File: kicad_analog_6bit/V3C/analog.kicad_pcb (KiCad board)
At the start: 2 copper layers, 50 x 23.2 mm, 35 parts, among them P1 Conn_02x06_Odd_Even, P2 Conn_01x04, P3 Conn_01x06, P6 Conn_01x01, P7 Conn_01x01, U1 MAX9108, U2 MAX9108, U3 MAX4610, U4 MAX5259EEE+, U5 MCP1754S-3302xCB, U6 TS5A3159ADBVR, U7 MAX9108-Comparator

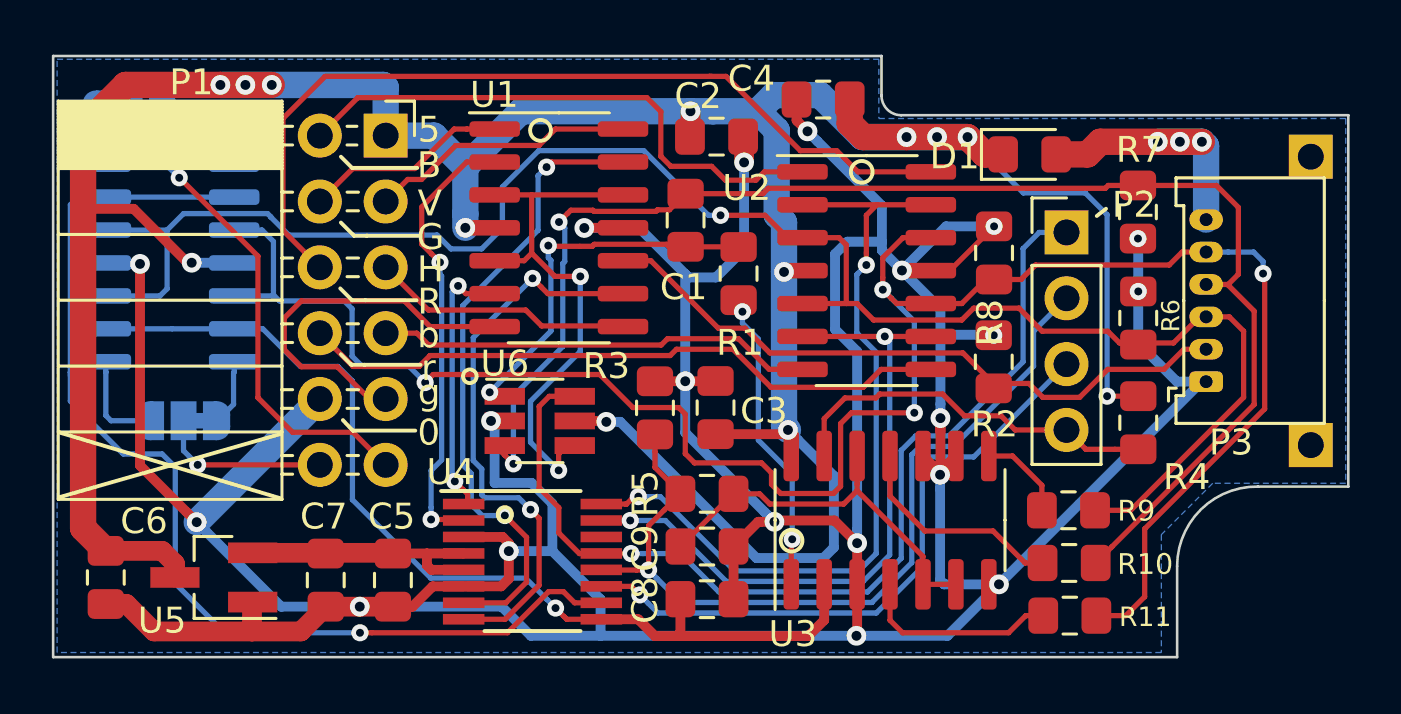
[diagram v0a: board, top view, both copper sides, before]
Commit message: V3 pcb plus some older alternatives
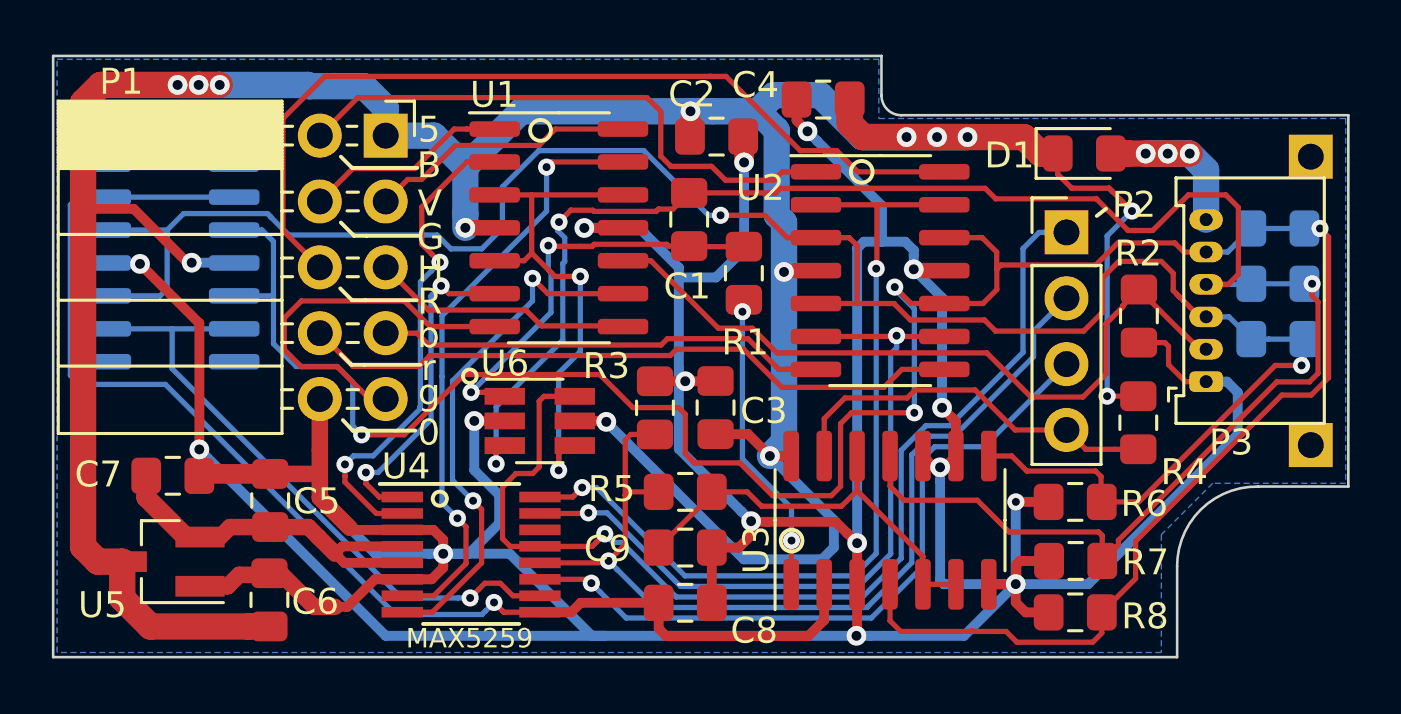
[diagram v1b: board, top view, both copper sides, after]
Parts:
- removed JP1, JP2: SolderJumper_3_Bridged12, Jumper:SolderJumper-3_P1.3mm_Bridged12_RoundedPad1.0x1.5mm
- P1: value Conn_02x06_Odd_Even -> Conn_02x05_Odd_Even; footprint Connector_PinSocket_2.54mm:PinSocket_2x06_P2.54mm_Horizontal -> Connector_PinSocket_2.54mm:PinSocket_2x05_P2.54mm_Horizontal
- R10, R11, R9: moved to B.Cu
- moved R11 17.0 mm to (74.8, 38.0), turned to 0 degrees
- moved R8 14.2 mm to (67.0, 52.8), turned to 180 degrees
- moved R7 13.7 mm to (67.0, 50.8), turned to 180 degrees
- moved R10 13.4 mm to (74.8, 40.1), turned to 0 degrees
- moved R9 10.4 mm to (74.8, 42.2), turned to 0 degrees
- moved R6 7.50 mm to (67.0, 48.5), turned to 180 degrees
- moved C7 7.14 mm to (32.1, 47.5), turned to 0 degrees
- moved C6 6.37 mm to (35.9, 52.3), turned to 90 degrees
- moved R2 5.87 mm to (69.4, 41.3), turned to 270 degrees
- moved C5 5.64 mm to (35.9, 48.5), turned to 90 degrees
- moved U4 2.38 mm to (43.7, 50.5)
- moved U5 2.12 mm to (31.7, 50.8)
- moved D1 2.11 mm to (67.3, 35.1)
- moved C8 0.85 mm to (51.9, 52.4)
- moved R5 0.84 mm to (51.9, 48.1)
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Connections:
- R10 pad 2: Net-(R10-Pad2) -> /AGREEN
- R11 pad 2: Net-(R11-Pad2) -> /ARED
- R9 pad 2: Net-(R9-Pad2) -> /ABLUE
- U3 pad 11: Net-(R10-Pad2) -> /AGREEN
- U3 pad 4: Net-(R11-Pad2) -> /ARED
- U3 pad 8: Net-(R9-Pad2) -> /ABLUE
- U7 pad 13: /SPARE -> /CLAMPLVL
- U7 pad 2: /SPARE -> /CLAMPLVL
- U7 pad 6: /CLAMPLVL -> /SPARE
- U7 pad 9: /CLAMPLVL -> /SPARE
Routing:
- net /ARED: track 80.0 -> 99.9 mm
- net /UV1: track 19.2 -> 0.00 mm, vias 1 -> 0
- net /AGREEN: track 56.0 -> 73.8 mm, vias 2 -> 3
- net /SPARE: track 42.2 -> 24.8 mm
- net /ABLUE: track 68.6 -> 81.3 mm, vias 1 -> 2
- net /CLAMPLVL: track 38.3 -> 49.8 mm
- net /GND: track 194.2 -> 203.5 mm, vias 20 -> 16
- net Net-(R10-Pad2): track 8.50 -> 0.00 mm
- net Net-(R11-Pad2): track 7.77 -> 0.00 mm
- net /VCC: track 129.0 -> 135.8 mm, vias 13 -> 14
- net /UV2: track 6.64 -> 0.00 mm, vias 1 -> 0
- net /VANALOG: track 10.1 -> 14.9 mm
- net /GPIO1_CLK: track 32.4 -> 36.6 mm
- net Net-(U7-Pad8): track 3.85 -> 0.00 mm
- net Net-(U7-Pad1): track 3.84 -> 0.00 mm
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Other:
- board text added: "Cut shorting links"
- board text added: "MAX5259"
- board text added: "Not Fitted"
- board text added: "Three level analog RGB/YUV & composite"
- board text added: "if R9-R11 required"
- board text removed: "Fit 10 way connector here"
- board text removed: "Fit for 12 way only"
- board text removed: "Three / Four level analog RGB/YUV & composite"
